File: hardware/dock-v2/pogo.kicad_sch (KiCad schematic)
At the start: 17 parts, among them J601 Pogo 7-pin, Q601 2N7002, Q602 2N7002, U601 TPD4E1U06DBVR, U602 SY6280AAC

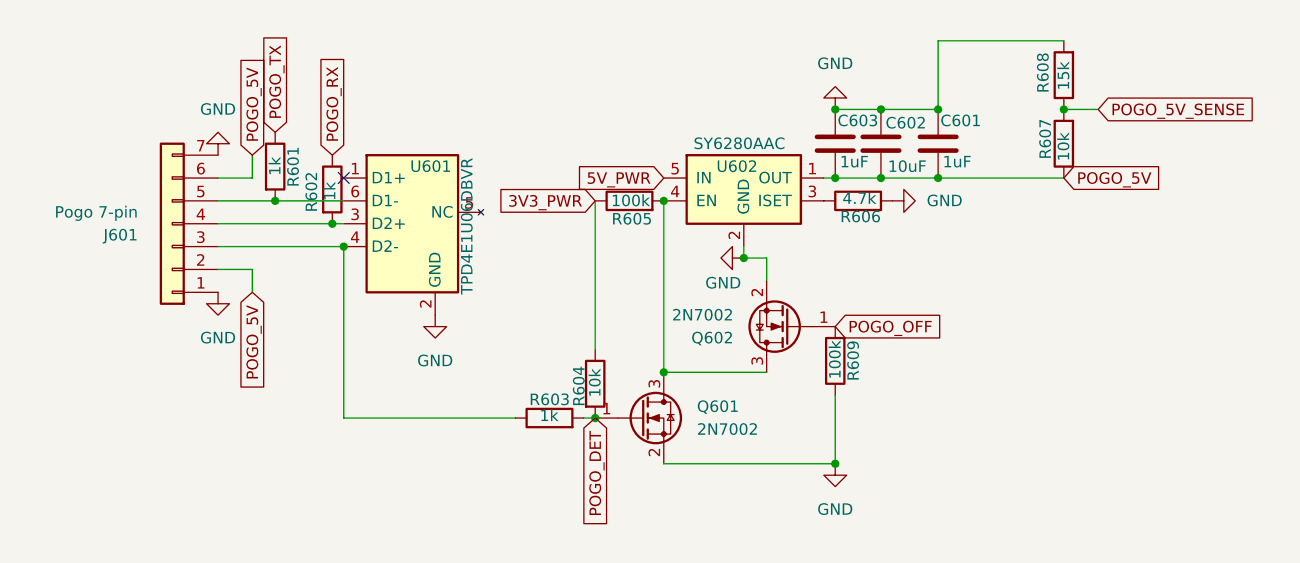
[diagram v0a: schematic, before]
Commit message: Dock v2 schematic: user's fixes (snapshot)
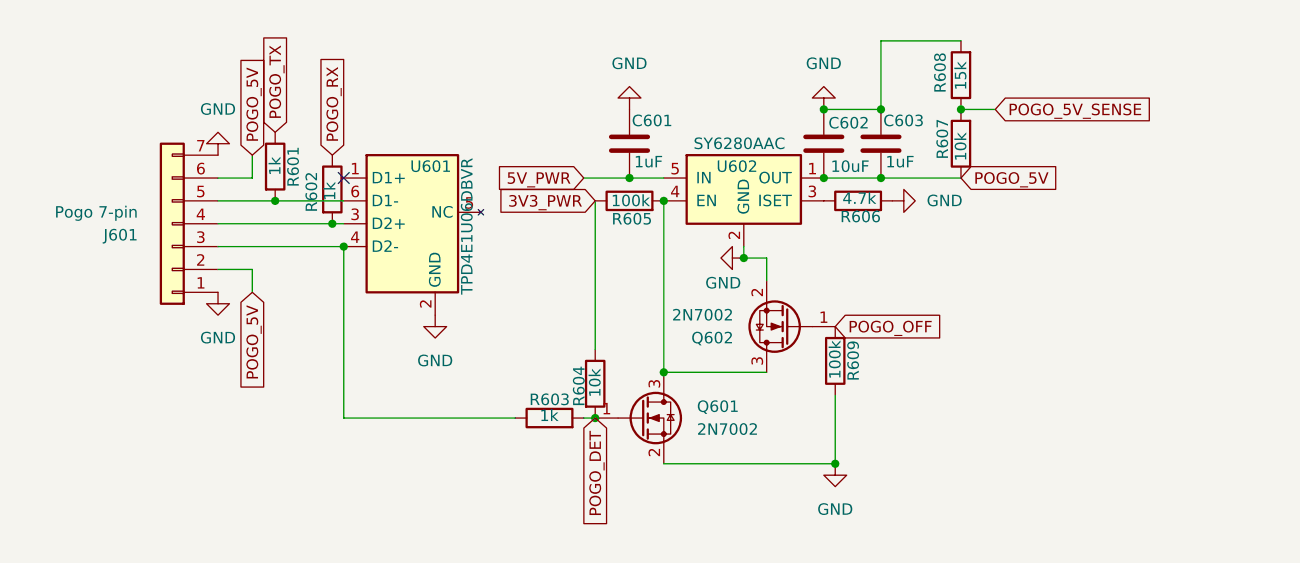
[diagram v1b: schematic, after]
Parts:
- removed C603: 1uF, Capacitor_SMD:C_0402_1005Metric, symbol Device:C
- added C601: 1uF, Capacitor_SMD:C_0402_1005Metric, symbol Device:C
- renumbered C601 to C603
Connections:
- net 5V_PWR: now also C601.2
- net GND: now also C601.1
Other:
- moved on the sheet: C602, C603, R607, R608

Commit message: Dock v2: placement and partial routing (user's work, snapshot)
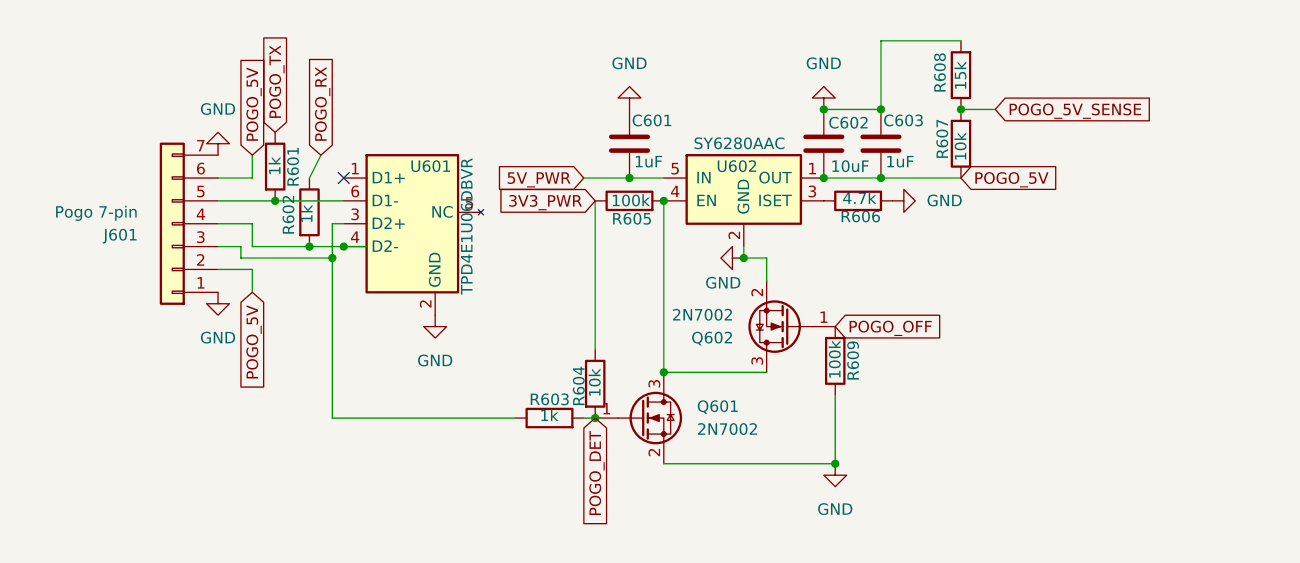
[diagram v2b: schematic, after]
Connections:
- net at J601.4 (Pin_4), R602.2: now also U601.4 (D2-); no longer U601.3 (D2+)
- net at J601.3 (Pin_3), R603.1: now also U601.3 (D2+); no longer U601.4 (D2-)
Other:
- moved on the sheet: R602
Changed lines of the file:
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@@
+	)
+	(junction
+		(at 114.3 21.59)
+		(diameter 0)
+		(color 0 0 0 0)
+	)
+	(junction
+		(at 114.3 29.21)
+		(diameter 0)
+		(color 0 0 0 0)
+	)
+	(junction
+		(at 129.54 21.59)
+		(diameter 0)
+		(color 0 0 0 0)
+	)
+	(junction
+		(at 57.15 36.83)
+		(diameter 0)
+		(color 0 0 0 0)
+	)
+	(junction
+		(at 115.57 60.96)
+		(diameter 0)
+		(color 0 0 0 0)
 	)
 	(junction
@@
 	)
 	(junction
-		(at 114.3 21.59)
-		(diameter 0)
-		(color 0 0 0 0)
-	)
-	(junction
-		(at 114.3 29.21)
-		(diameter 0)
-		(color 0 0 0 0)
-	)
-	(junction
-		(at 129.54 21.59)
-		(diameter 0)
-		(color 0 0 0 0)
-	)
-	(junction
-		(at 115.57 60.96)
-		(diameter 0)
-		(color 0 0 0 0)
-	)
-	(junction
 		(at 88.9 55.88)
 		(diameter 0)
@@
 	)
 	(junction
-		(at 59.69 34.29)
+		(at 59.69 38.1)
 		(diameter 0)
 		(color 0 0 0 0)
@@
 	(wire
 		(pts
+			(xy 57.15 29.21) (xy 58.42 26.67)
+		)
+		(stroke
+			(width 0)
+			(type default)
+		)
+	)
+	(wire
+		(pts
 			(xy 87.63 55.88) (xy 88.9 55.88)
 		)
@@
 	(wire
 		(pts
+			(xy 59.69 38.1) (xy 59.69 34.29)
+		)
+		(stroke
+			(width 0)
+			(type default)
+		)
+	)
+	(wire
+		(pts
 			(xy 105.41 38.1) (xy 105.41 36.83)
 		)
@@
 	(wire
 		(pts
+			(xy 50.8 34.29) (xy 46.99 34.29)
+		)
+		(stroke
+			(width 0)
+			(type default)
+		)
+	)
+	(wire
+		(pts
 			(xy 88.9 31.75) (xy 88.9 48.26)
 		)
@@
 	(wire
 		(pts
-			(xy 60.96 55.88) (xy 80.01 55.88)
+			(xy 49.53 38.1) (xy 59.69 38.1)
 		)
 		(stroke
@@
 	(wire
 		(pts
-			(xy 60.96 36.83) (xy 60.96 55.88)
+			(xy 59.69 34.29) (xy 60.96 34.29)
+		)
+		(stroke
+			(width 0)
+			(type default)
+		)
+	)
+	(wire
+		(pts
+			(xy 50.8 36.83) (xy 50.8 34.29)
 		)
 		(stroke
@@
 	(wire
 		(pts
-			(xy 46.99 34.29) (xy 59.69 34.29)
-		)
-		(stroke
-			(width 0)
-			(type default)
-		)
-	)
-	(wire
-		(pts
 			(xy 114.3 21.59) (xy 120.65 21.59)
 		)
@@
 	(wire
 		(pts
-			(xy 59.69 34.29) (xy 60.96 34.29)
+			(xy 57.15 36.83) (xy 60.96 36.83)
 		)
 		(stroke
@@
 	(wire
 		(pts
+			(xy 46.99 36.83) (xy 49.53 36.83)
+		)
+		(stroke
+			(width 0)
+			(type default)
+		)
+	)
+	(wire
+		(pts
 			(xy 133.35 21.59) (xy 129.54 21.59)
 		)
@@
 	(wire
 		(pts
+			(xy 59.69 55.88) (xy 80.01 55.88)
+		)
+		(stroke
+			(width 0)
+			(type default)
+		)
+	)
+	(wire
+		(pts
+			(xy 50.8 36.83) (xy 57.15 36.83)
+		)
+		(stroke
+			(width 0)
+			(type default)
+		)
+	)
+	(wire
+		(pts
+			(xy 49.53 36.83) (xy 49.53 38.1)
+		)
+		(stroke
+			(width 0)
+			(type default)
+		)
+	)
+	(wire
+		(pts
 			(xy 50.8 41.91) (xy 50.8 39.37)
 		)
@@
 	(wire
 		(pts
+			(xy 59.69 38.1) (xy 59.69 55.88)
+		)
+		(stroke
+			(width 0)
+			(type default)
+		)
+	)
+	(wire
+		(pts
 			(xy 129.54 13.97) (xy 120.65 13.97)
 		)
@@
 	(wire
 		(pts
-			(xy 46.99 36.83) (xy 60.96 36.83)
+			(xy 63.5 36.83) (xy 60.96 36.83)
 		)
 		(stroke
@@
 	(global_label "POGO_RX"
 		(shape input)
-		(at 59.69 26.67 90)
+		(at 58.42 26.67 90)
 		(fields_autoplaced yes)
 		(effects
@@
 		)
 		(property "Intersheetrefs" "${INTERSHEET_REFS}"
-			(at 59.69 15.0367 90)
+			(at 58.42 15.0367 90)
 			(hide yes)
 			(show_name no)
@@
 	(symbol
 		(lib_id "Device:R")
-		(at 59.69 30.48 0)
+		(at 57.15 33.02 0)
 		(unit 1)
 		(body_style 1)
@@
 		(dnp no)
 		(property "Reference" "R602"
-			(at 57.404 33.02 90)
+			(at 54.864 35.56 90)
 			(show_name no)
 			(do_not_autoplace no)
@@
 		)
 		(property "Value" "1k"
-			(at 59.436 31.75 90)
+			(at 56.896 34.29 90)
 			(show_name no)
 			(do_not_autoplace no)
@@
 		)
 		(property "Footprint" "Resistor_SMD:R_0402_1005Metric"
-			(at 59.69 30.48 0)
+			(at 57.15 33.02 0)
 			(hide yes)
 			(show_name no)
@@
 		)
 		(property "Datasheet" ""
-			(at 59.69 30.48 0)
+			(at 57.15 33.02 0)
 			(hide yes)
 			(show_name no)
@@
 		)
 		(property "Description" "Resistor"
-			(at 59.69 30.48 0)
+			(at 57.15 33.02 0)
 			(hide yes)
 			(show_name no)
@@
 		)
 		(property "LCSC" "C11702"
-			(at 59.69 30.48 0)
+			(at 57.15 33.02 0)
 			(hide yes)
 			(show_name no)
@@
 		)
 		(property "Note" "RX series"
-			(at 63.25 34.29 0)
-			(hide yes)
-			(show_name no)
+			(at 60.71 36.83 0)
+			(hide yes)
+			(show_name no)
